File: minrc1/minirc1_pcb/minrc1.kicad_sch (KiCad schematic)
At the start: 18 parts, among them J3 Conn_01x04, J4 Conn_01x04, U1 DRV8837D, U2 DRV8837D, U3 DRV8837D, U4 DRV8837D, U5 ESP32S3

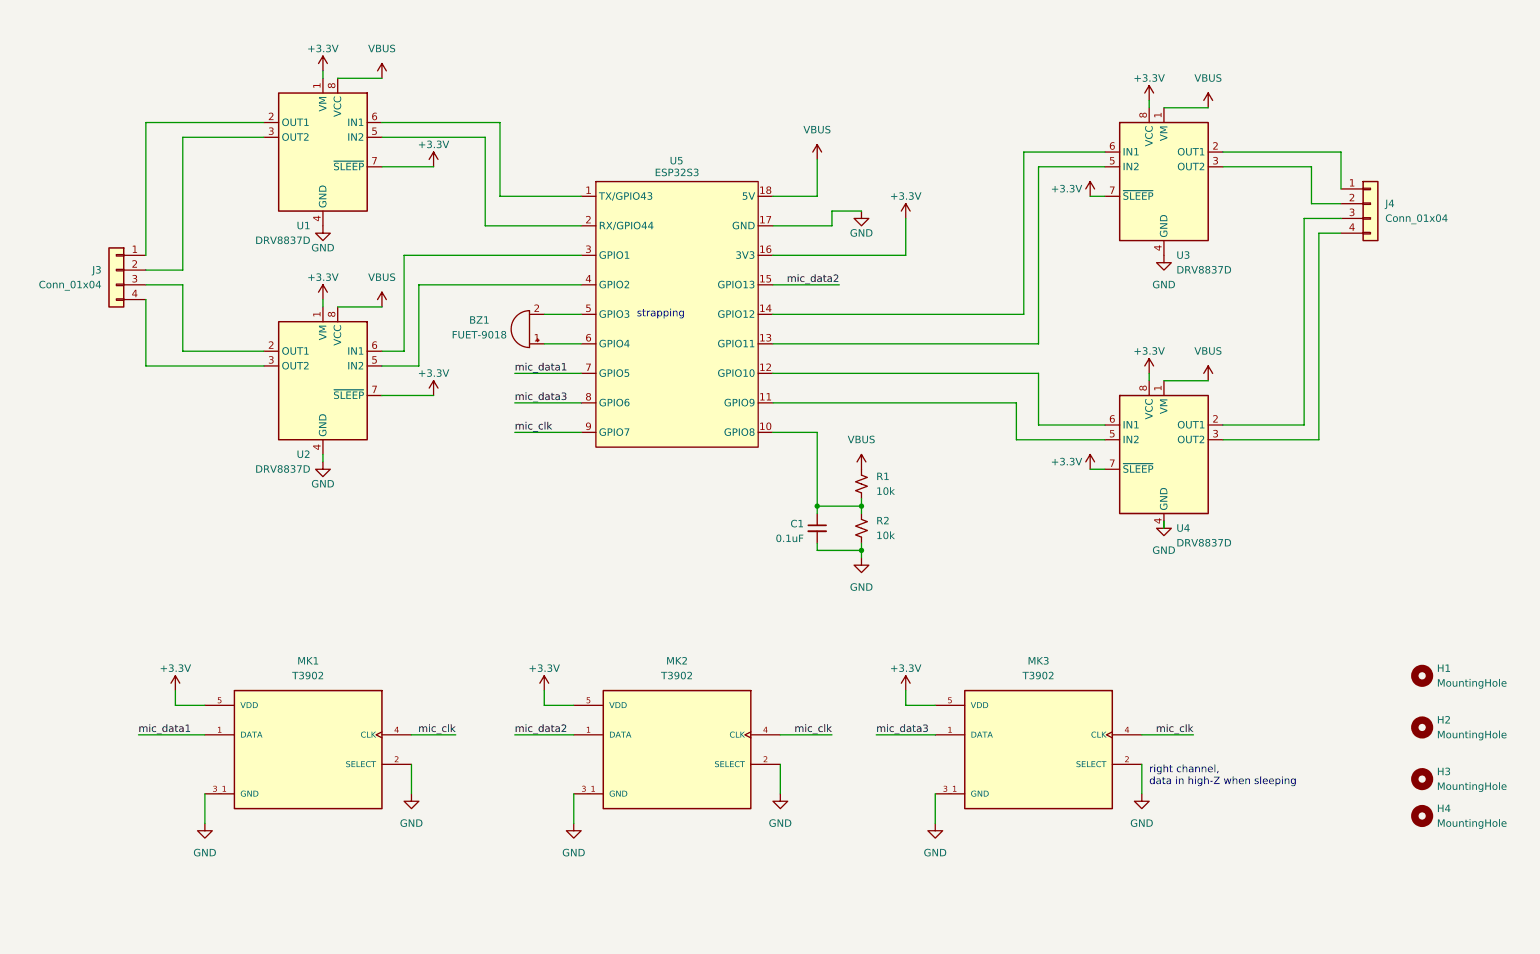
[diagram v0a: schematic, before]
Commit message: finish turtlebot
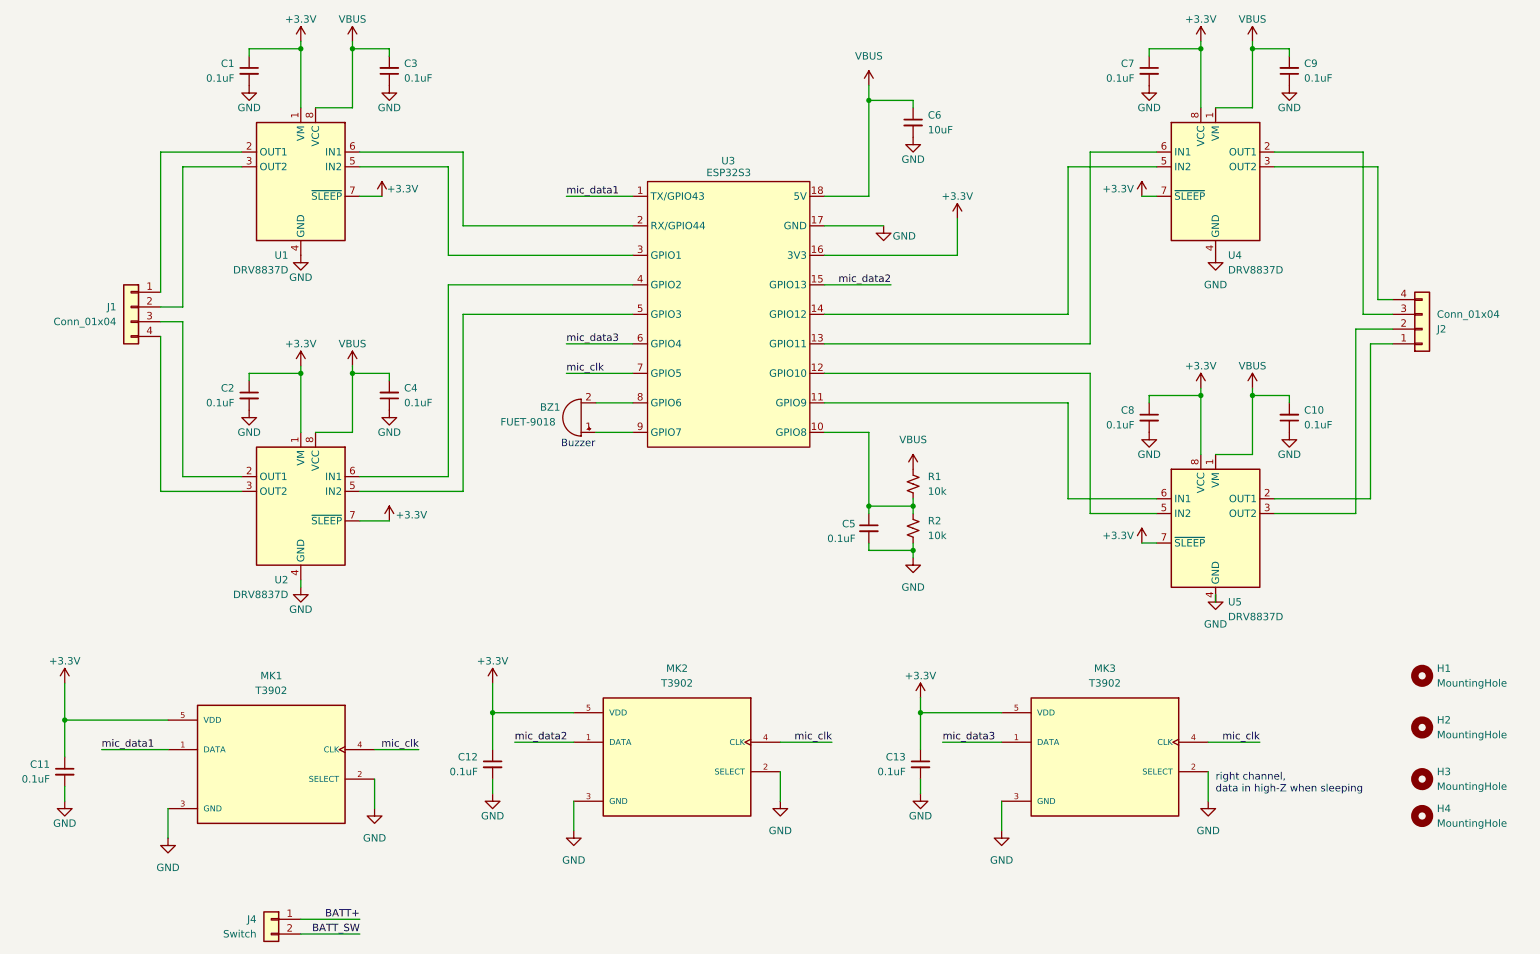
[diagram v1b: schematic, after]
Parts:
- added C1, C10, C11, C12, C13, C2, C3, C4, C7, C8, C9: 0.1uF, Resistor_SMD:R_0402_1005Metric, symbol Device:C_Small
- added C6: 10uF, Resistor_SMD:R_0402_1005Metric, symbol Device:C_Small
- added J4: Switch, Connector_PinHeader_2.54mm:PinHeader_1x02_P2.54mm_Vertical, symbol Connector_Generic:Conn_01x02
- C5: renamed from C1; footprint (none) -> Resistor_SMD:R_0402_1005Metric
- renumbered J3 to J1, J4 to J2, U5 to U3, U3 to U4, U4 to U5
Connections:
- net +3.3V: now also C1.1, C11.1, C12.1, C13.1, C2.1, C7.1, C8.1
- net GND: now also MK1.3 (GND), MK2.3 (GND), MK3.3 (GND), C1.2, C10.1, C11.2, C12.2, C13.2, C2.2, C3.1, C4.1, C6.2, C7.2, C8.2, C9.1; no longer MK1.3_1 (GND), MK1.3_2 (GND), MK2.3_1 (GND), MK2.3_2 (GND), MK3.3_1 (GND), MK3.3_2 (GND)
- net VBUS: now also C10.2, C3.2, C4.2, C6.1, C9.2
- net mic_clk: now also U3.7 (GPIO5); no longer U3.9 (GPIO7)
- net mic_data1: now also U3.1 (TX/GPIO43); no longer U3.7 (GPIO5)
- net mic_data3: now also U3.6 (GPIO4); no longer U3.8 (GPIO6)
- net at BZ1.1 (+): now also U3.9 (GPIO7); no longer U3.6 (GPIO4)
- net at BZ1.2 (-): now also U3.8 (GPIO6); no longer U3.5 (GPIO3)
- net at U1.5 (IN2): now also U3.3 (GPIO1); no longer U3.2 (RX/GPIO44)
- net at U1.6 (IN1): now also U3.2 (RX/GPIO44); no longer U3.1 (TX/GPIO43)
- net at U2.5 (IN2): now also U3.5 (GPIO3); no longer U3.4 (GPIO2)
- net at U2.6 (IN1): now also U3.4 (GPIO2); no longer U3.3 (GPIO1)
- net at U3.11 (GPIO9): now also U5.6 (IN1); no longer U5.5 (IN2)
- net at U3.12 (GPIO10): now also U5.5 (IN2); no longer U5.6 (IN1)
- net at U3.13 (GPIO11): now also U4.6 (IN1); no longer U4.5 (IN2)
- net at U3.14 (GPIO12): now also U4.5 (IN2); no longer U4.6 (IN1)
- net at U5.2 (OUT1): now also J2.1 (Pin_1); no longer J2.3 (Pin_3)
- net at U5.3 (OUT2): now also J2.2 (Pin_2); no longer J2.4 (Pin_4)
- net at U4.2 (OUT1): now also J2.3 (Pin_3); no longer J2.1 (Pin_1)
- net at U4.3 (OUT2): now also J2.4 (Pin_4); no longer J2.2 (Pin_2)
- new net BATT+: J4.1 (Pin_1)
- new net BATT_SW: J4.2 (Pin_2)
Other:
- note added: "Buzzer"
- note removed: "strapping"
- moved on the sheet: BZ1, C5, J1, J2, MK1, MK2, MK3, R1, R2, U1, U2, U3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
